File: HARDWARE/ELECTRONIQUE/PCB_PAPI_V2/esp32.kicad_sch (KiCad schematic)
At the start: 26 parts, among them J2 636101111001, Y2 LFXTAL069527REEL

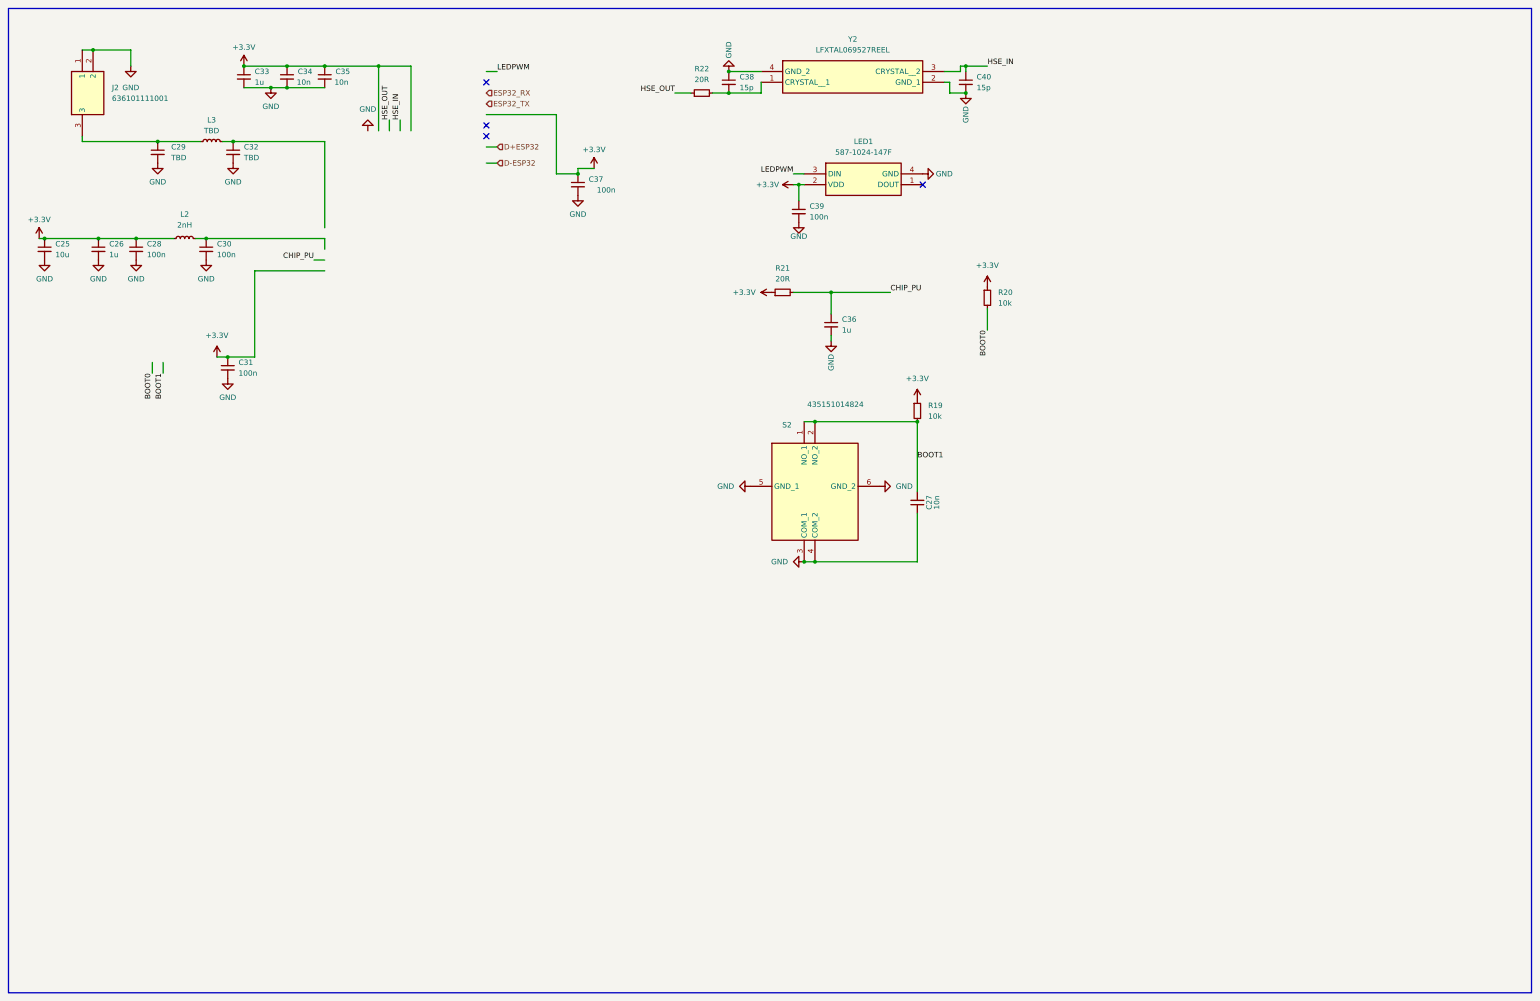
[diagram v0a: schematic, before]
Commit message: up
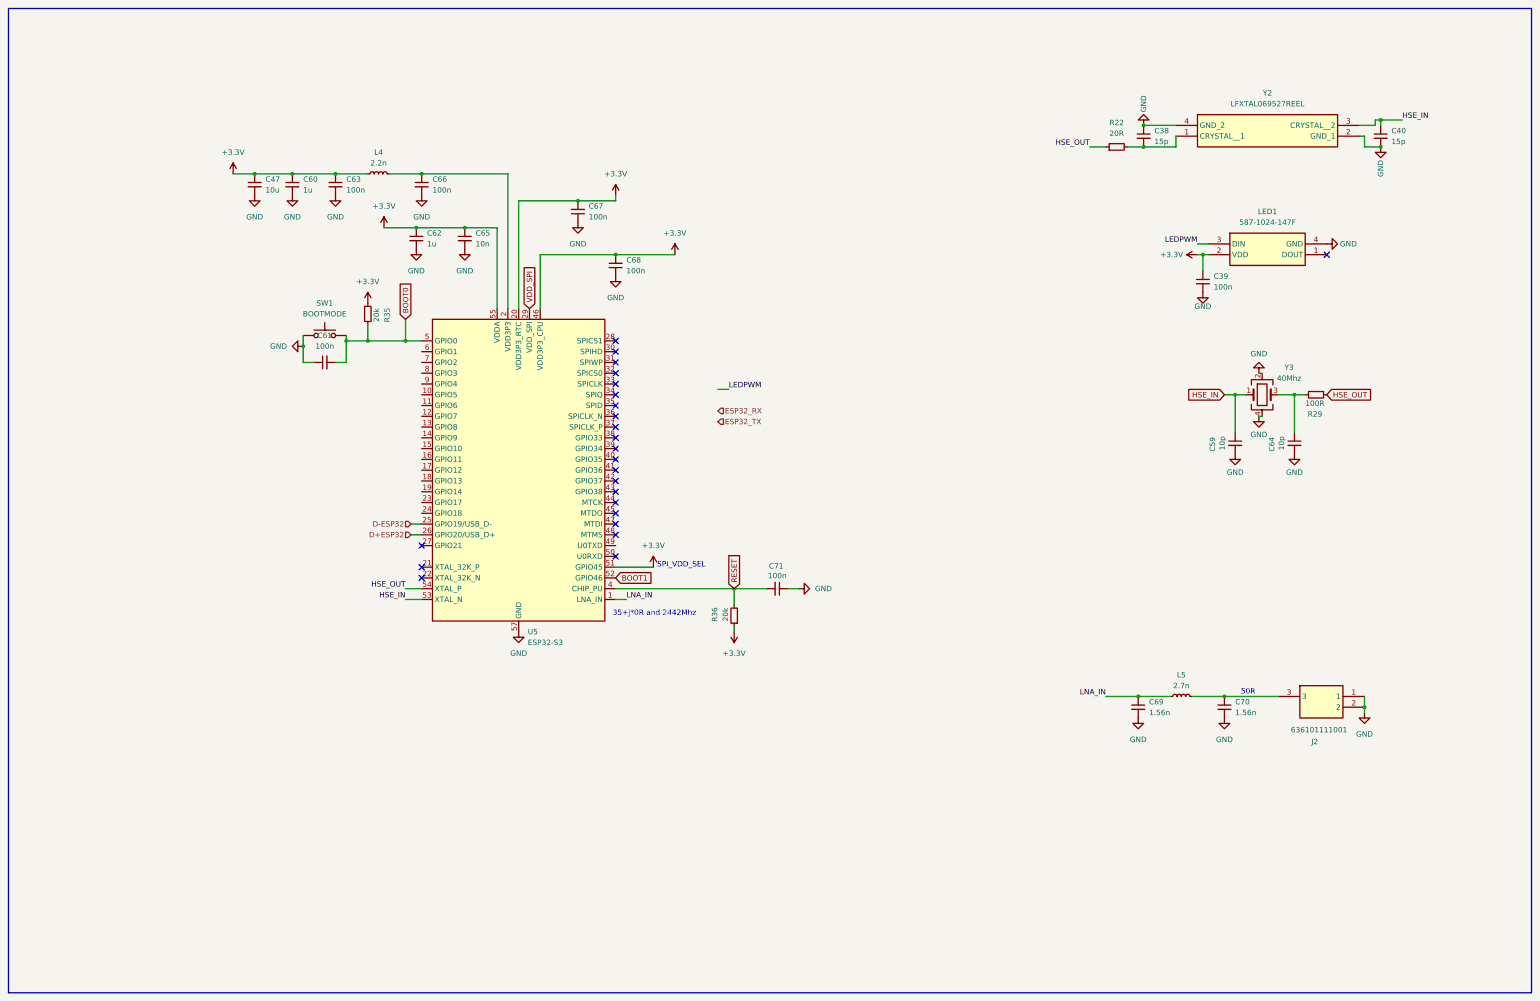
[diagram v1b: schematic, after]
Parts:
- removed C25: 10u, Capacitor_SMD:C_0402_1005Metric, symbol Device:C_Small
- removed C26, C33, C36: 1u, Capacitor_SMD:C_0402_1005Metric, symbol Device:C_Small
- removed C27, C34, C35: 10n, samacsys:C_0201_custom, symbol Device:C_Small
- removed C28, C30: 100n, Capacitor_SMD:C_0201_0603Metric, symbol Device:C_Small
- removed C29, C32: TBD, Capacitor_SMD:C_0402_1005Metric, symbol Device:C_Small
- removed C31, C37: 100n, samacsys:C_0201_custom, symbol Device:C_Small
- removed L2: 2nH, Inductor_SMD:L_0402_1005Metric, symbol Device:L_Small
- removed L3: TBD, Inductor_SMD:L_0402_1005Metric, symbol Device:L_Small
- removed R19, R20: 10k, Resistor_SMD:R_0201_0603Metric, symbol Device:R_Small
- removed R21: 20R, samacsys:R_0201_custom, symbol Device:R_Small
- removed S2: 435151014824, samacsys:435151014824, symbol samacsys:435151014824
- added C47: 10u, Capacitor_SMD:C_0402_1005Metric_Pad0.74x0.62mm_HandSolder, symbol Device:C_Small
- added C59, C64: 10p, Capacitor_SMD:C_0201_0603Metric_Pad0.64x0.40mm_HandSolder, symbol Device:C_Small
- added C60, C62: 1u, Capacitor_SMD:C_0402_1005Metric_Pad0.74x0.62mm_HandSolder, symbol Device:C_Small
- added C61, C63, C66, C67, C68, C71: 100n, Capacitor_SMD:C_0201_0603Metric_Pad0.64x0.40mm_HandSolder, symbol Device:C_Small
- added C65: 10n, Capacitor_SMD:C_0201_0603Metric_Pad0.64x0.40mm_HandSolder, symbol Device:C_Small
- added C69, C70: 1.56n, Capacitor_SMD:C_0402_1005Metric_Pad0.74x0.62mm_HandSolder, symbol Device:C_Small
- added L4: 2.2n, Inductor_SMD:L_0603_1608Metric, symbol Device:L_Small
- added L5: 2.7n, Inductor_SMD:L_0603_1608Metric, symbol Device:L_Small
- added R29: 100R, Resistor_SMD:R_0201_0603Metric_Pad0.64x0.40mm_HandSolder, symbol Device:R_Small
- added R35, R36: 20k, Resistor_SMD:R_0201_0603Metric_Pad0.64x0.40mm_HandSolder, symbol Device:R_Small
- added SW1: BOOTMODE, samacsys:KXT341LHS, symbol Switch:SW_Omron_B3FS
- added U5: ESP32-S3, Package_DFN_QFN:QFN-56-1EP_7x7mm_P0.4mm_EP4x4mm, symbol MCU_Espressif:ESP32-S3
- added Y3: 40Mhz, samacsys:LFXTAL069527REEL, symbol Device:Crystal_GND24
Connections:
- net +3.3V: now also C47.1, C60.1, C62.1, C63.1, C65.1, C67.2, C68.2, L4.1, R35.1, R36.1, U5.20 (VDD3P3_RTC), U5.46 (VDD3P3_CPU), U5.51 (GPIO45), U5.55 (VDDA), U5.56 (VDDA)
- net BOOT0: now also C61.2, R35.2, SW1.2, U5.5 (GPIO0)
- net BOOT1: now also U5.52 (GPIO46)
- net D+ESP32: now also U5.26 (GPIO20/USB_D+)
- net D-ESP32: now also U5.25 (GPIO19/USB_D-)
- net GND: now also C47.2, C59.2, C60.2, C61.1, C62.2, C63.2, C64.2, C65.2, C66.2, C67.1, C68.1, C69.2, C70.2, C71.1, SW1.1, U5.57 (GND), Y3.2, Y3.4
- net HSE_IN: now also C59.1, U5.53 (XTAL_N), Y3.1
- net HSE_OUT: now also R29.1, U5.54 (XTAL_P)
- net at J2.3: now also C70.1, L5.2
- new net: C64.1, R29.2, Y3.3
- new net: C66.1, L4.2, U5.2 (VDD3P3), U5.3 (VDD3P3)
- new net LNA_IN: C69.1, L5.1, U5.1 (LNA_IN)
- new net RESET: C71.2, R36.2, U5.4 (CHIP_PU)
- new net VDD_SPI: U5.29 (VDD_SPI)
- no-connect marks 4 -> 24
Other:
- note added: "35+j*0R and 2442Mhz"
- note added: "50R"
- note added: "SPI_VDD_SEL"
- moved on the sheet: C38, C39, C40, J2, LED1, R22, Y2
